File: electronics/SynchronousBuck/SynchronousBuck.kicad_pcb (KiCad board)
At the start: 4 copper layers, 90 x 81 mm, 55 parts, among them J101 Conn_01x02, J102 Conn_01x04_Male, J103 Conn_01x02, J104 Conn_01x02, Q101 BSC070N10NS5, Q102 BSC067N06LS3G, U101 LM5116MH

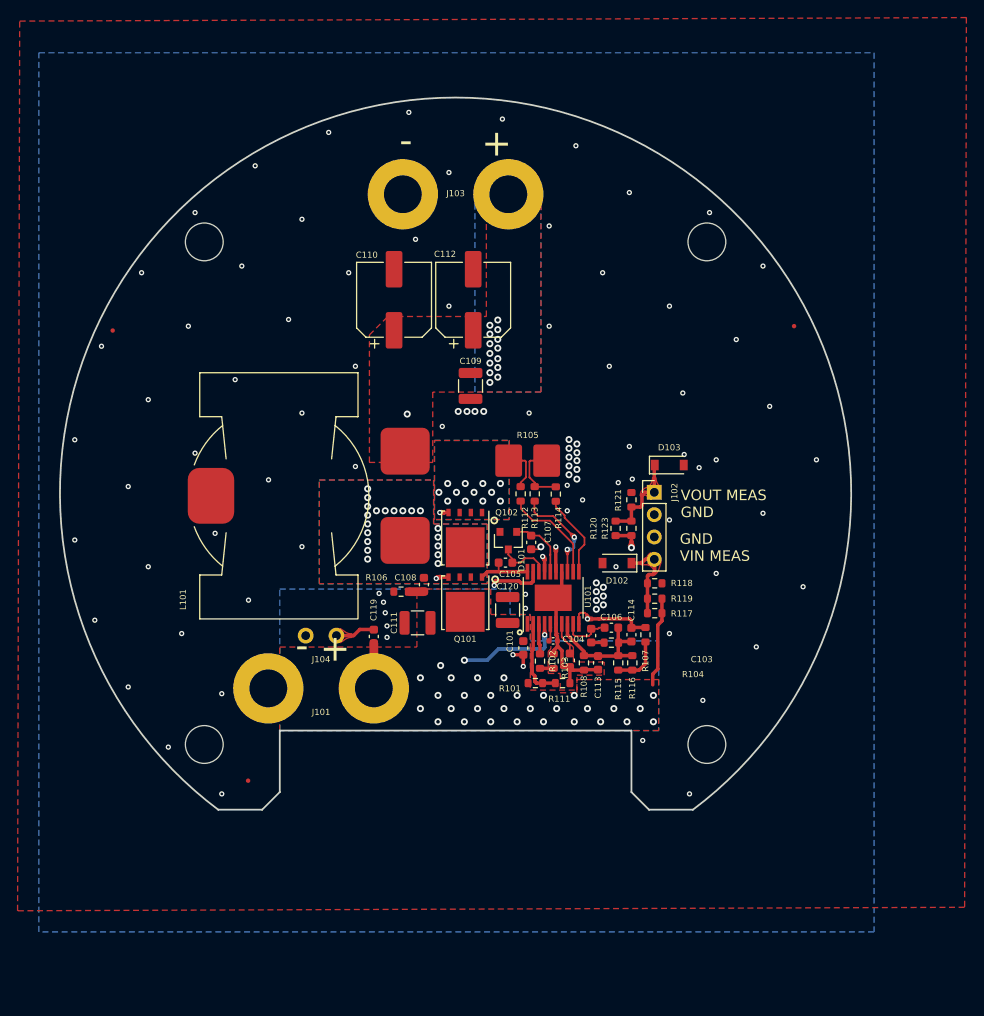
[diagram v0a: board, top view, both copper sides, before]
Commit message: Folder restructuring
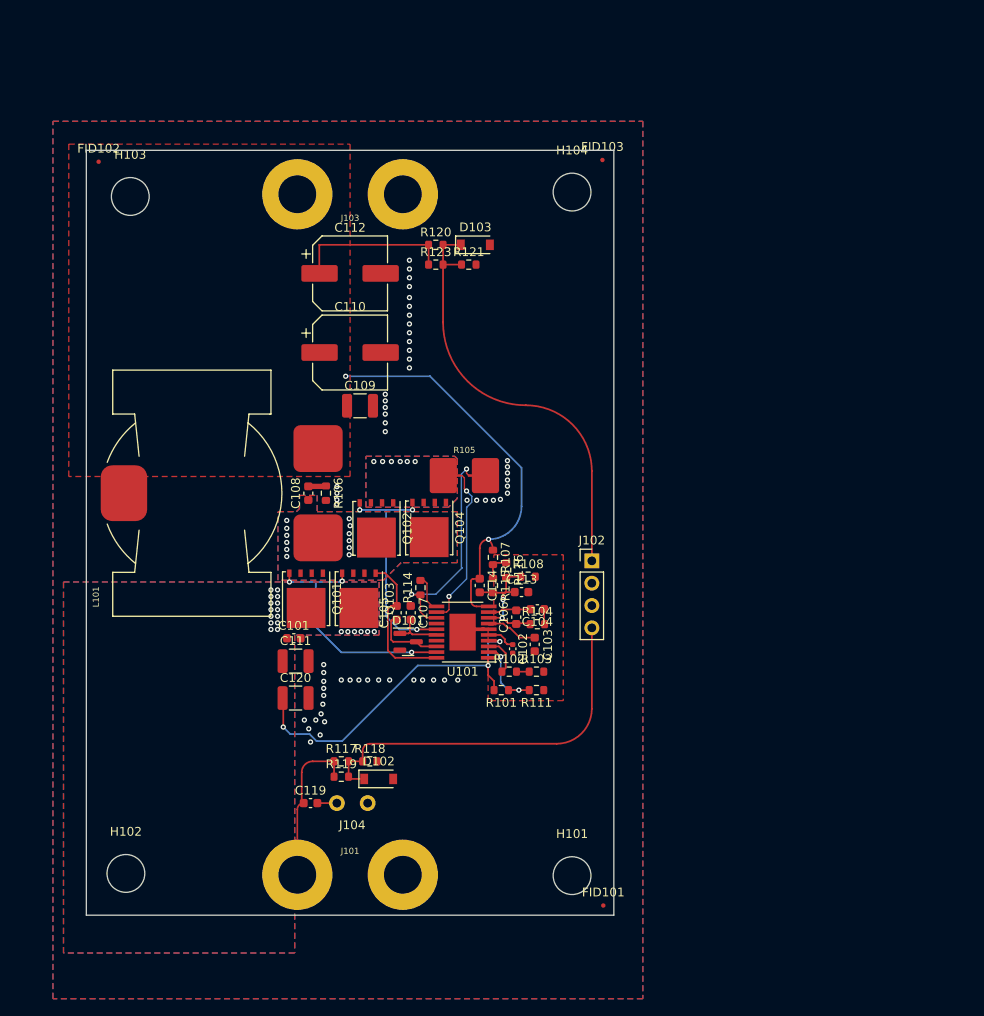
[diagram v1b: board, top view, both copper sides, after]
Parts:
- removed G***: LOGO, SynchronousBuck:SubLogo
- removed R112, R113: 100, Resistor_SMD:R_0603_1608Metric
- added NT101: NetTie_2, NetTie:NetTie-2_SMD_Pad0.5mm, F.Cu at (102.7, 115.5)
- added Q103: BSC070N10NS5, Package_TO_SOT_SMD:TDSON-8-1, F.Cu at (89.0, 112.0)
- added Q104: BSC067N06LS3G, Package_TO_SOT_SMD:TDSON-8-1, F.Cu at (97.0, 104.0)
- J101, J103: footprint PCBDecals:2xM4 -> SynchronousBuck:2xM4
- J104: footprint Misc:1x2_3.5_pinHeader -> SynchronousBuck:1x2_3.5_pinHeader
- L101: footprint Misc:WE-HCF -> SynchronousBuck:WE-HCF
- R105: footprint PCBDecals:LR2512_3WLOW_SHUNT -> SynchronousBuck:R_2512_6332Metric_SHUNT
- moved FID102 81.3 mm to (59.4, 62.3), turned to 0 degrees
- moved FID103 59.0 mm to (116.7, 62.1), turned to 0 degrees
- moved FID101 42.8 mm to (116.8, 146.9), turned to 0 degrees
- moved R119 41.0 mm to (87.0, 132.2), turned to 0 degrees
- moved R117 39.4 mm to (87.0, 130.5), turned to 0 degrees
- moved R118 38.2 mm to (90.2, 130.5)
- moved R120 38.2 mm to (97.8, 71.8), turned to 0 degrees
- moved R123 37.4 mm to (97.8, 74.0), turned to 0 degrees
- moved D102 36.6 mm to (91.2, 132.5), turned to 0 degrees
- moved D103 33.4 mm to (102.2, 71.8)
- moved R121 32.5 mm to (101.5, 74.0), turned to 0 degrees
- moved C101 26.1 mm to (81.6, 116.5), turned to 0 degrees
- moved C120 26.1 mm to (81.8, 123.3), turned to 0 degrees
- moved J101 21.5 mm to (88.0, 143.4), turned to 180 degrees
- moved H101 21.4 mm to (113.2, 143.5), turned to 0 degrees
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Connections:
- net Net-(C106-Pad1) renamed /FB
- net Net-(Q102-Pad1) renamed /ShuntTop
- C102 pad 2: GND -> GNDA
- C103 pad 2: GND -> GNDA
- C113 pad 2: GND -> GNDA
- D101 pad 2: Net-(D101-Pad2) -> unconnected-(D101-Pad2)
- L101 pad 3: GND -> unconnected-(L101-Pad3)
- R103 pad 2: GND -> GNDA
- R108 pad 2: GND -> GNDA
- R111 pad 1: GND -> GNDA
- U101 pad 12: Net-(R112-Pad2) -> Net-(R105-Pad2)
- U101 pad 13: Net-(R113-Pad2) -> Net-(R105-Pad3)
- U101 pad 17: /VOUT -> GND
- U101 pad 6: GND -> GNDA
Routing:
- net /VOUT: track 118.2 -> 64.5 mm, vias 18 -> 2
- net Net-(D103-Pad1): track 10.1 -> 49.1 mm
- net Net-(D102-Pad1): track 9.50 -> 44.2 mm
- net VCC: track 27.8 -> 58.4 mm, vias 32 -> 23
- net GND: track 24.3 -> 0.00 mm, vias 100 -> 58
- net Net-(R105-Pad3): track 5.79 -> 24.6 mm, vias 0 -> 2
- net Net-(R105-Pad2): track 3.27 -> 18.7 mm, vias 0 -> 2
- net /HO: track 14.8 -> 27.3 mm, vias 2 -> 3
- net Net-(R112-Pad2): track 11.6 -> 0.00 mm
- net Net-(R113-Pad2): track 11.6 -> 0.00 mm, vias 2 -> 0
- net /SW: track 6.49 -> 17.1 mm, vias 20 -> 12
- net /LO: track 19.6 -> 25.4 mm, vias 2 -> 3
- net Net-(U101-Pad11): track 9.62 -> 4.22 mm
- net Net-(R107-Pad2): track 5.88 -> 3.16 mm
- net Net-(C119-Pad2): track 4.55 -> 2.22 mm
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- added copper zone on In1.Cu, net /ShuntTop
- added copper zone on In2.Cu, net /ShuntTop
- added copper zone on F.Cu, net GNDA
- removed copper zone on B.Cu, net /VOUT
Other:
- board size 90 x 81 mm -> 60 x 87 mm
- net class Default removed
- board text removed: "+ -"
- board text removed: "GND VIN MEAS"
- board text removed: "SN:"
- board text removed: "Synchronous Buck V1.0 Findersee 23/21"
- board text removed: "VOUT MEAS GND"
